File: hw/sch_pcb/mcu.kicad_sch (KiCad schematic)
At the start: 60 parts, among them IC1 MAX14502AETL+, IC2 TMUX1574DYYR, J22 HEADER_2x03, J9 SD_Card-FPS009-4200-0, Q4 BC817-25, SW2 MCU_RST, SW3 SW_Push, U10 ATMEGA1284P-AU, U11 PCF85263A, U3 ISL21080DIH309, U6 AT24CS64-SSHM, Y1 8 MHz, Y2 ABS07-120-32.768KHZ-T

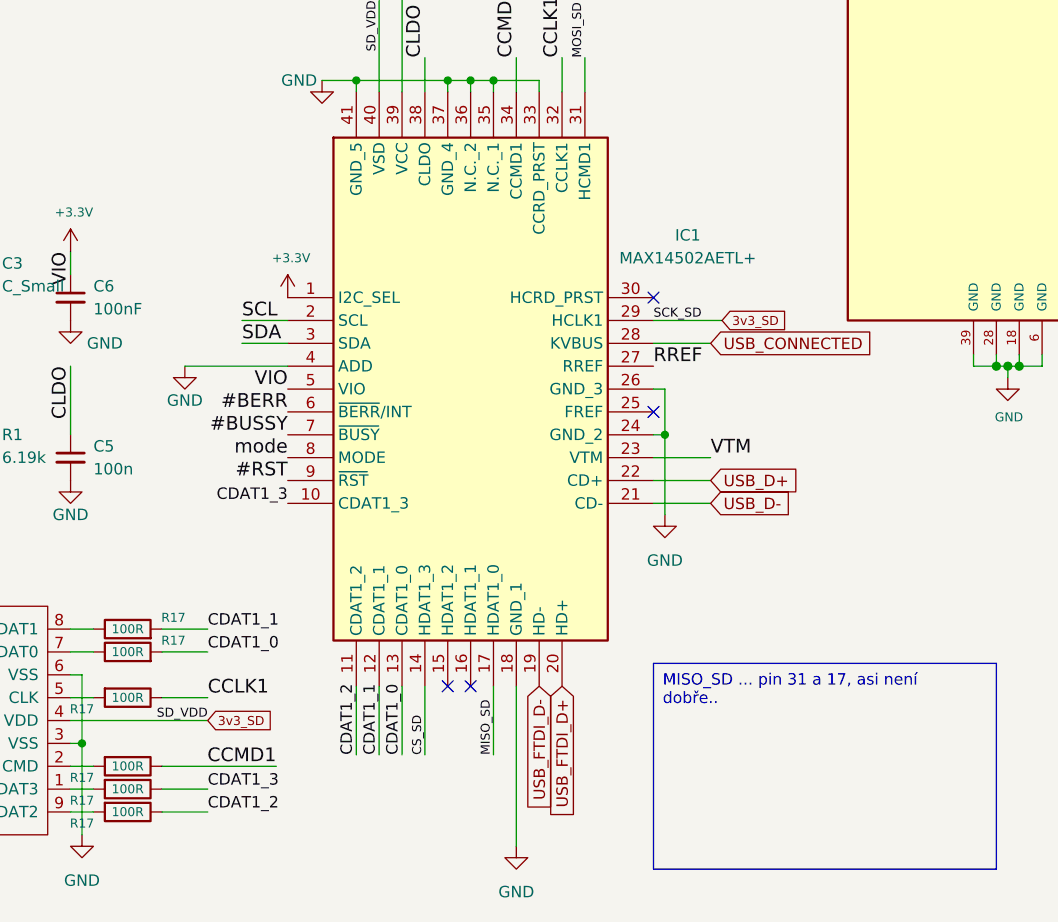
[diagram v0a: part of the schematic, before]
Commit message: WIP
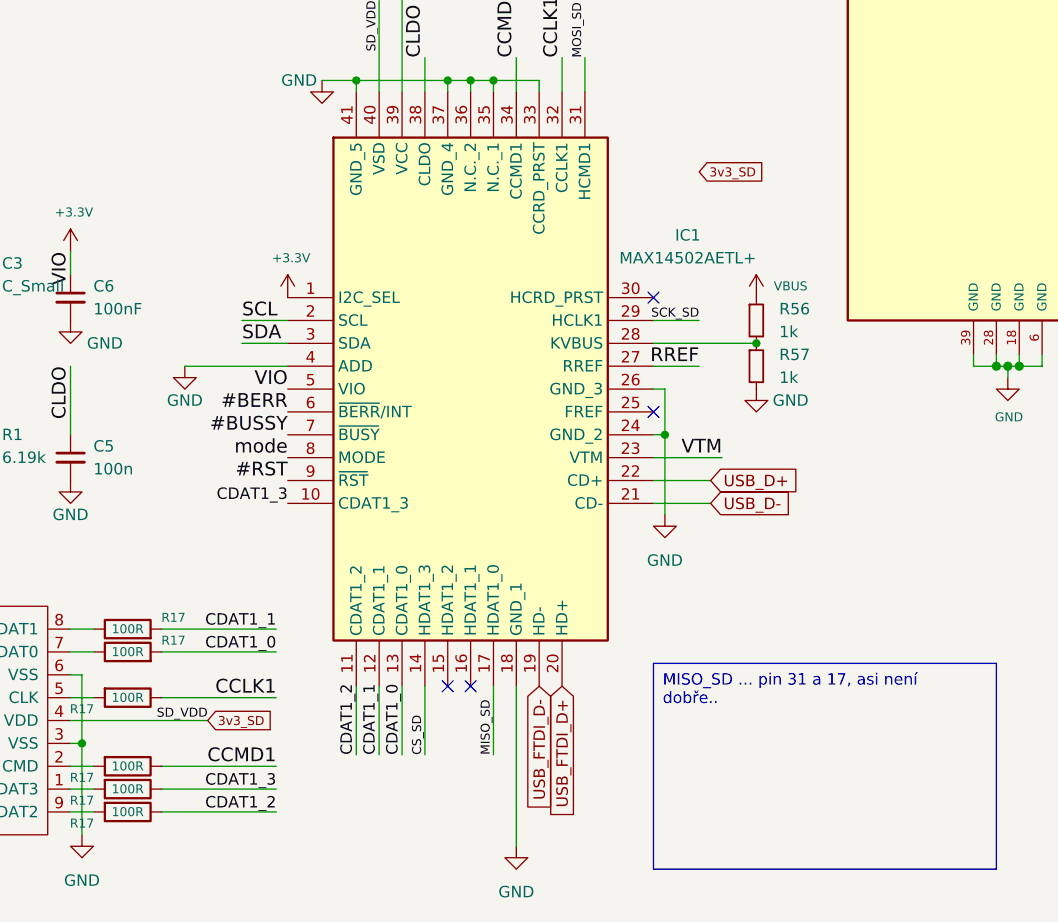
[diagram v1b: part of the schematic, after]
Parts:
- added R56, R57: 1k, Resistor_SMD:R_0805_2012Metric, symbol Device:R_Small
- R40, R78: footprint (none) -> Resistor_SMD:R_0805_2012Metric
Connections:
- net 3v3_SD: no longer IC1.29 (HCLK1), IC2.11 (S3A)
- net GND: now also R57.2
- net USB_CONNECTED: no longer names the net of IC1.28 (KVBUS)
- net USB_CONNECTED: now also R56.2, R57.1
- new net SCK_SD: IC1.29 (HCLK1), IC2.11 (S3A)
- new net VBUS: R56.1
